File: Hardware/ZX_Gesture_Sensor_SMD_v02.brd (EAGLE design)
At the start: 57.3 x 19.1 mm, 51 parts, among them Q1 MMBT2222A, Q2 MOSFET-NCHANNEL2N7002PW, U1 PIC16F1823-14PINTSSOP, U2 MCP6021T-E/OT, U3 DMC2700UDM, U4 DMC2700UDM, U6 TSOP57238TT1

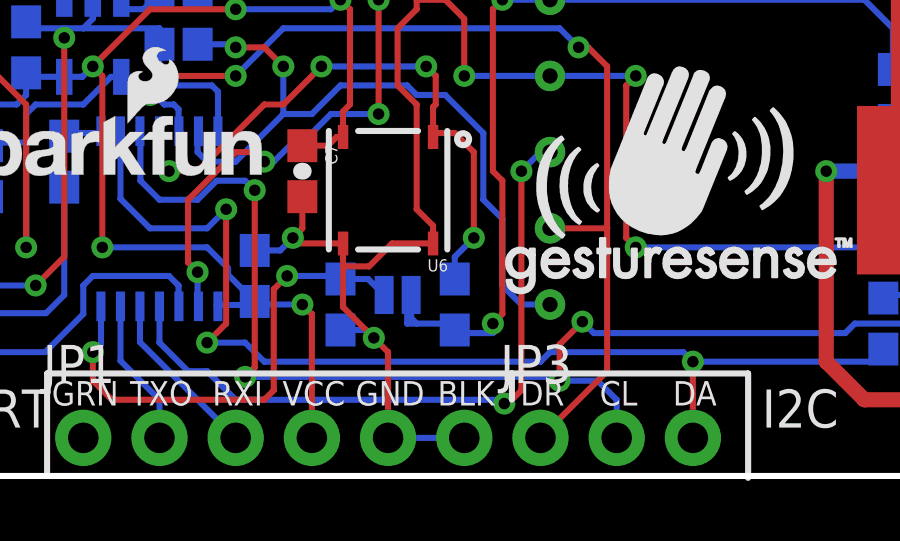
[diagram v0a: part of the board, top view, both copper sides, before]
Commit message: Updated Board Files per QC
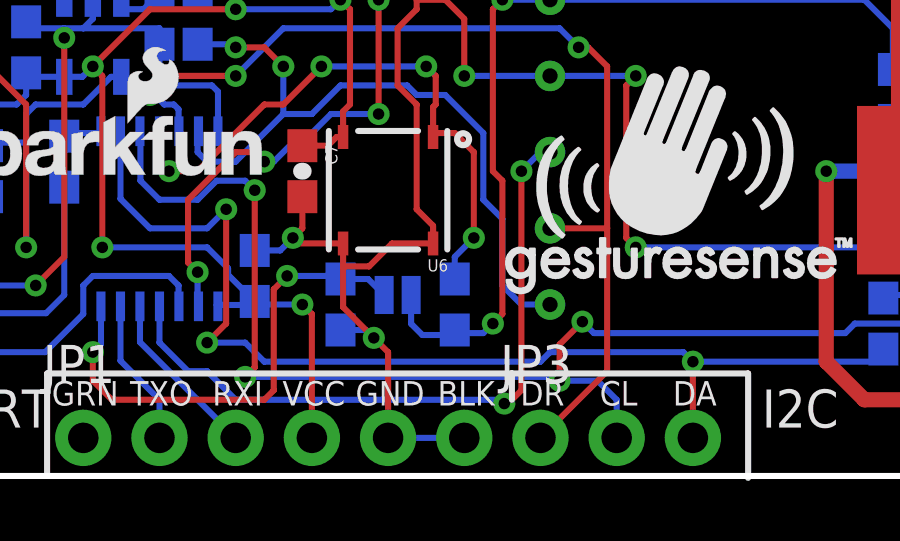
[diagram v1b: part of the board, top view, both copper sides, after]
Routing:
- net VCC: track 106.9 -> 106.3 mm
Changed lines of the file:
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@@
 <wire x1="23.241" y1="6.9215" x2="23.241" y2="6.7065" width="0.2032" layer="16"/>
 <wire x1="23.241" y1="6.7065" x2="24.13" y2="5.8175" width="0.2032" layer="16"/>
-<wire x1="29.3425" y1="6.0325" x2="29.3425" y2="5.265" width="0.2032" layer="16"/>
-<wire x1="29.3425" y1="5.265" x2="29.5275" y2="5.08" width="0.2032" layer="16"/>
-<wire x1="29.5275" y1="5.08" x2="30.5825" y2="5.08" width="0.2032" layer="16"/>
-<wire x1="30.5825" y1="5.08" x2="30.7975" y2="4.865" width="0.2032" layer="16"/>
 <wire x1="27.305" y1="15.5575" x2="27.305" y2="12.3825" width="0.2032" layer="1"/>
 <wire x1="26.9875" y1="15.875" x2="27.305" y2="15.5575" width="0.2032" layer="1"/>
@@
 <wire x1="24.13" y1="5.715" x2="24.13" y2="5.8175" width="0.2032" layer="16"/>
 <via x="25.7175" y="5.715" extent="1-16" drill="0.381"/>
-<wire x1="29.21" y1="5.08" x2="29.21" y2="5.3975" width="0.2032" layer="16"/>
-<wire x1="29.5275" y1="5.08" x2="29.21" y2="5.08" width="0.2032" layer="16"/>
-<wire x1="30.7975" y1="4.7625" x2="32.0675" y2="4.7625" width="0.2032" layer="16"/>
 <wire x1="30.7975" y1="4.7625" x2="30.7975" y2="4.865" width="0.2032" layer="16"/>
-<wire x1="32.0675" y1="5.08" x2="32.0675" y2="4.7625" width="0.2032" layer="16"/>
 <wire x1="32.385" y1="5.3975" x2="32.0675" y2="5.08" width="0.2032" layer="1"/>
 <wire x1="32.385" y1="9.8425" x2="32.385" y2="5.3975" width="0.2032" layer="1"/>
@@
 <wire x1="50.165" y1="10.6925" x2="50.4825" y2="10.375" width="0.2032" layer="16"/>
 <wire x1="50.1015" y1="11.1125" x2="50.165" y2="11.049" width="0.2032" layer="16"/>
+<wire x1="29.3425" y1="6.0325" x2="29.3425" y2="5.0745" width="0.2032" layer="16"/>
+<wire x1="29.3425" y1="5.0745" x2="29.718" y2="4.699" width="0.2032" layer="16"/>
+<wire x1="29.718" y1="4.699" x2="30.6315" y2="4.699" width="0.2032" layer="16"/>
+<wire x1="30.6315" y1="4.699" x2="30.7975" y2="4.865" width="0.2032" layer="16"/>
+<wire x1="30.7975" y1="4.7625" x2="31.75" y2="4.7625" width="0.2032" layer="16"/>
+<wire x1="31.75" y1="4.7625" x2="32.0675" y2="5.08" width="0.2032" layer="16"/>
 </signal>
 <signal name="GND">
